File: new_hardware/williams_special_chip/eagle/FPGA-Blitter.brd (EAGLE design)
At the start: 68.6 x 68.6 mm, 5 parts, among them IC1 SPECIAL_CHIP, IC2 IDTQS32X861

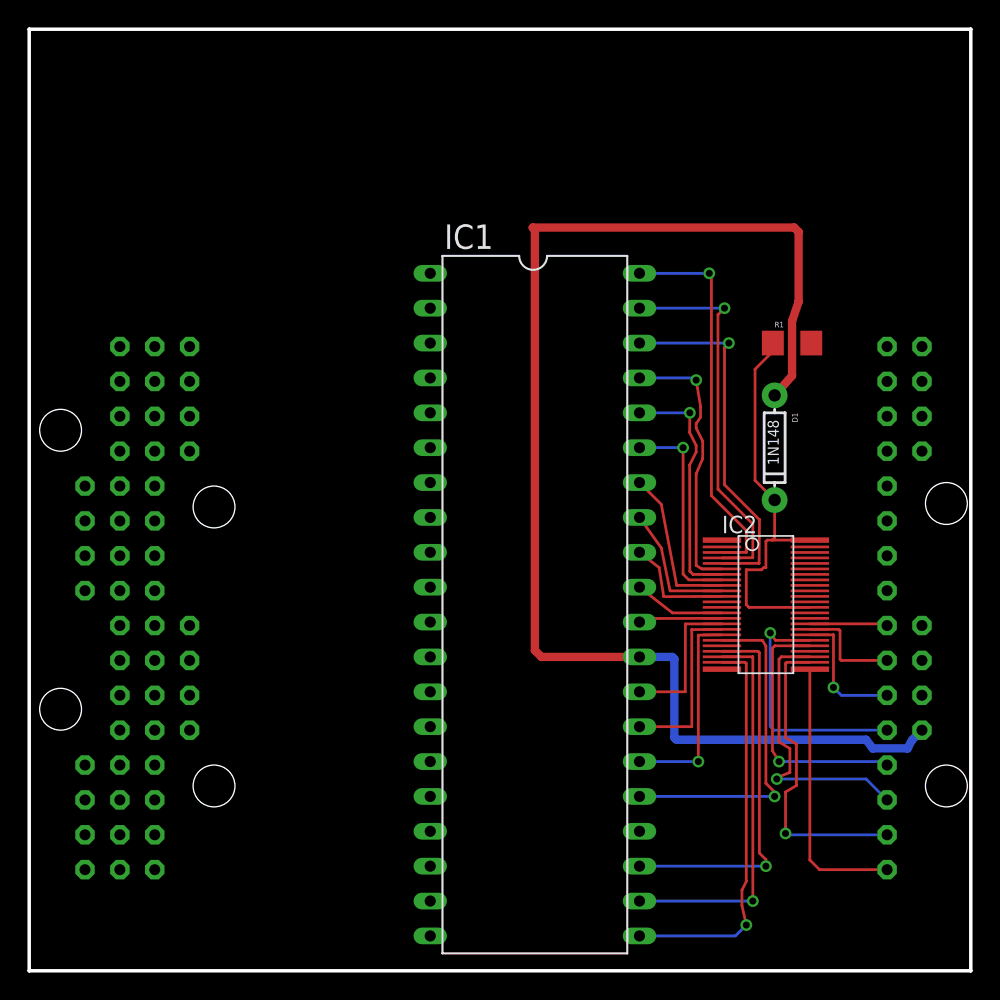
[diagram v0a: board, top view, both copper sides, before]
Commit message: gotta just verify pins chosen and this is ready for production
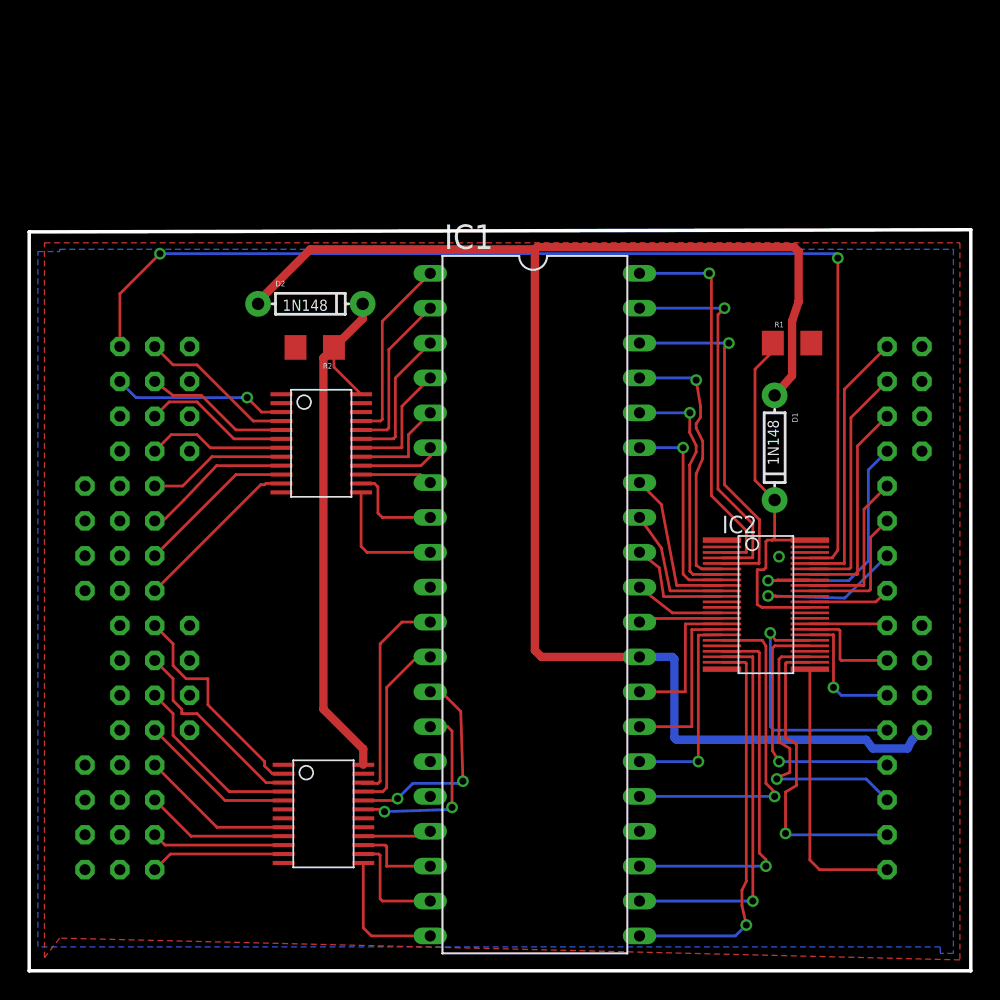
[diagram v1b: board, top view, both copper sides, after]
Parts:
- added D2: 1N148, SparkFun:DIODE-1N4148
- added IC3, IC4: IDTQS3861, mpo:TSSOP24
- added R2: 10k, SparkFun:1206
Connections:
- removed net N$1: U$2.AL_5V
- removed net N$2: U$2.AU_5V
- removed net N$3: U$2.BL_5V
- new net !BA-BS_3V3: IC3.8, U$2.B4
- new net !HALT_3V3: IC3.7, U$2.B3
- new net !HTCF_3V3: IC3.5, U$2.B1
- new net !RESET_3V3: IC2.41, U$2.C3
- new net !TCF_3V3: IC3.4, U$2.B0
- new net !WINH_3V3: IC2.45, U$2.A15
- new net 4MHZ_3V3: IC2.40, U$2.C4
- new net A11_3V3: IC2.38, U$2.C6
- new net A12_3V3: IC2.39, U$2.C5
- new net A13_3V3: IC2.42, U$2.C2
- new net A14_3V3: IC2.43, U$2.C1
- new net A15_3V3: IC2.44, U$2.C0
- new net A3_3V3: IC4.10, U$2.B14
- new net A4_3V3: IC4.11, U$2.B15
- new net D0_3V3: IC4.8, U$2.B12
- new net D1_3V3: IC4.4, U$2.B10
- new net D2_3V3: IC4.3, U$2.B9
- new net D3_3V3: IC4.2, U$2.B8
- new net D4_3V3: IC3.11, U$2.B7
- new net D5_3V3: IC3.10, U$2.B6
- new net D6_3V3: IC3.9, U$2.B5
- new net D7_3V3: IC3.6, U$2.B2
- new net E_3V3: IC3.3, U$2.A14
- new net N$4: D2.C, IC3.24, IC4.24, R2.1
- new net R/!W_3V3: IC4.9, U$2.B13
- new net U/!L_3V3: IC4.5, U$2.B11
- net !BA-BS: now also IC3.16
- net !E: now also IC3.21
- net !HALT: now also IC3.17
- net !HTCF: now also IC3.19
- net !TCF: now also IC3.20
- net A3: now also IC4.14
- net A4: now also IC4.13
- net D0: now also IC4.16
- net D1: now also IC4.20
- net D2: now also IC4.21
- net D3: now also IC4.22
- net D4: now also IC3.13
- net D5: now also IC3.14
- net D6: now also IC3.15
- net D7: now also IC3.18
- net GND: now also IC3.12, IC3.23, IC4.12, IC4.23, R2.2
- net R/!W: now also IC4.15
- net U/!L: now also IC4.19
- net VCC: now also D2.A
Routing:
- net !WINH_3V3: track 0.00 -> 81.1 mm, vias 0 -> 2
- net N$4: track 0.00 -> 40.2 mm
- net A15_3V3: track 0.00 -> 19.6 mm
- net !RESET_3V3: track 0.00 -> 19.5 mm, vias 0 -> 1
- net VCC: track 98.1 -> 116.8 mm
- net A14_3V3: track 0.00 -> 17.7 mm
- net D3_3V3: track 0.00 -> 16.1 mm
- net A13_3V3: track 0.00 -> 15.9 mm
- net D3: track 0.00 -> 15.7 mm
- net D1: track 0.00 -> 15.7 mm, vias 0 -> 2
- net D2_3V3: track 0.00 -> 14.2 mm
- net U/!L: track 0.00 -> 13.9 mm, vias 0 -> 2
- net !E: track 0.00 -> 13.7 mm
- net D1_3V3: track 0.00 -> 13.2 mm
- net D2: track 0.00 -> 13.2 mm
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- added copper zone on layer 1, net GND
- added copper zone on layer 16, net GND
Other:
- board size 68.6 x 68.6 mm -> 68.6 x 54 mm
